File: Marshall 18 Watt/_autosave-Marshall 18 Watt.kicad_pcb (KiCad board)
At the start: 2 copper layers, 37 parts, among them J1 LOW, J2 HIGH, J3 Conn_01x03_Socket, J4 Heater, U1 ECC83, U2 ECC83, U3 EL84, U4 EL84

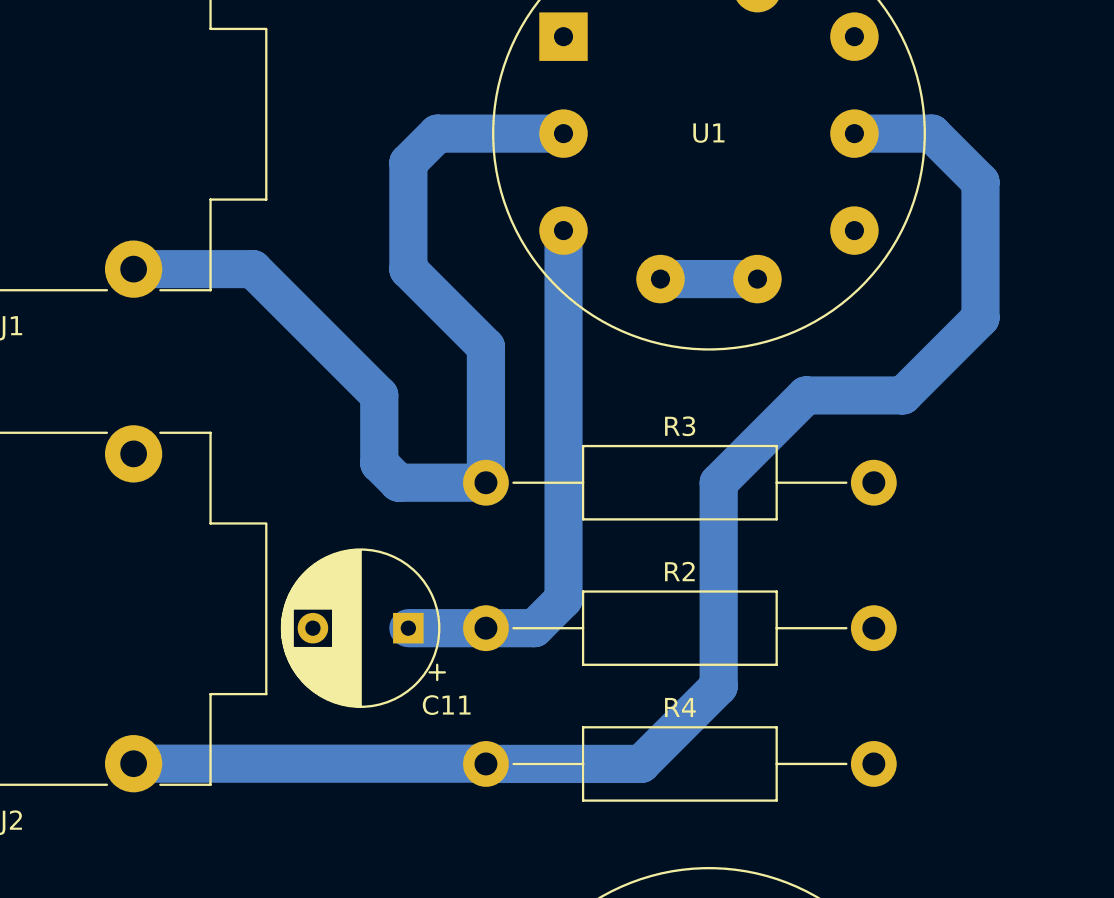
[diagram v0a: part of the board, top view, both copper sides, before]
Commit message: Update 11_03_25
add fender champ
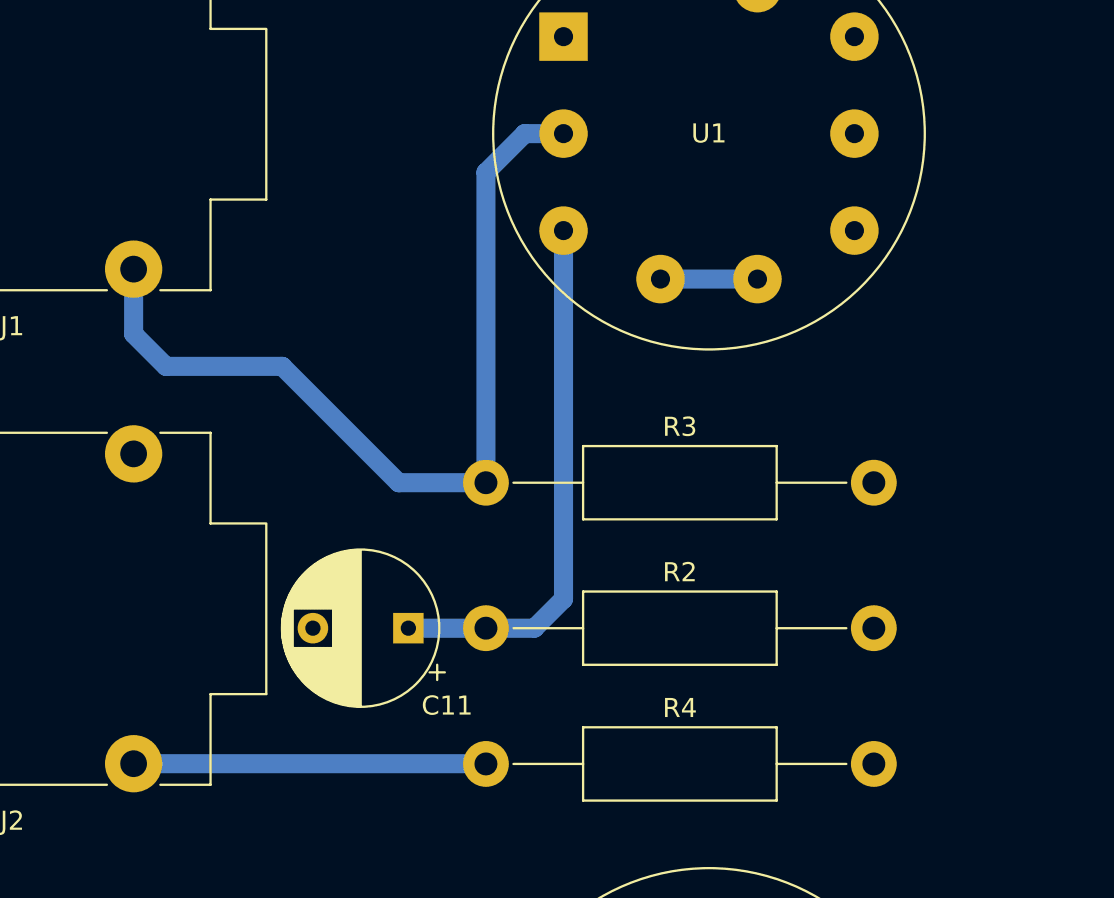
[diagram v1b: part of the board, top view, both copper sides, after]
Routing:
- net Net-(U1A-G): track 75.1 -> 18.5 mm
- net Net-(U1B-G): track 52.4 -> 46.2 mm
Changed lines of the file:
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@@
     )
   )
-  (segment (start 63.5 52.324) (end 66.04 52.324) (width 2) (layer "B.Cu") (net 6))
-  (segment (start 66.04 52.324) (end 67.564 50.8) (width 2) (layer "B.Cu") (net 6))
-  (segment (start 59.436 52.324) (end 63.5 52.324) (width 2) (layer "B.Cu") (net 6))
-  (segment (start 67.564 50.8) (end 67.564 31.496) (width 2) (layer "B.Cu") (net 6))
-  (segment (start 51.295 33.515) (end 57.912 40.132) (width 2) (layer "B.Cu") (net 10))
-  (segment (start 60.96 26.416) (end 67.564 26.416) (width 2) (layer "B.Cu") (net 10))
-  (segment (start 58.928 44.704) (end 63.5 44.704) (width 2) (layer "B.Cu") (net 10))
-  (segment (start 59.436 33.528) (end 59.436 27.94) (width 2) (layer "B.Cu") (net 10))
-  (segment (start 57.912 43.688) (end 58.928 44.704) (width 2) (layer "B.Cu") (net 10))
-  (segment (start 57.912 40.132) (end 57.912 43.688) (width 2) (layer "B.Cu") (net 10))
-  (segment (start 59.436 27.94) (end 60.96 26.416) (width 2) (layer "B.Cu") (net 10))
-  (segment (start 63.5 44.704) (end 63.5 37.592) (width 2) (layer "B.Cu") (net 10))
-  (segment (start 63.5 37.592) (end 59.436 33.528) (width 2) (layer "B.Cu") (net 10))
-  (segment (start 45.043 33.515) (end 51.295 33.515) (width 2) (layer "B.Cu") (net 10))
-  (segment (start 71.628 59.436) (end 75.692 55.372) (width 2) (layer "B.Cu") (net 11))
-  (segment (start 85.344 40.132) (end 89.408 36.068) (width 2) (layer "B.Cu") (net 11))
-  (segment (start 75.692 44.704) (end 80.264 40.132) (width 2) (layer "B.Cu") (net 11))
-  (segment (start 80.264 40.132) (end 85.344 40.132) (width 2) (layer "B.Cu") (net 11))
-  (segment (start 86.868 26.416) (end 82.804 26.416) (width 2) (layer "B.Cu") (net 11))
-  (segment (start 63.487 59.423) (end 63.5 59.436) (width 2) (layer "B.Cu") (net 11))
-  (segment (start 89.408 28.956) (end 86.868 26.416) (width 2) (layer "B.Cu") (net 11))
-  (segment (start 89.408 36.068) (end 89.408 28.956) (width 2) (layer "B.Cu") (net 11))
-  (segment (start 45.043 59.423) (end 63.487 59.423) (width 2) (layer "B.Cu") (net 11))
-  (segment (start 63.5 59.436) (end 71.628 59.436) (width 2) (layer "B.Cu") (net 11))
-  (segment (start 75.692 55.372) (end 75.692 44.704) (width 2) (layer "B.Cu") (net 11))
-  (segment (start 72.644 34.036) (end 77.724 34.036) (width 2) (layer "B.Cu") (net 19))
+  (segment (start 63.5 52.324) (end 59.436 52.324) (width 1) (layer "B.Cu") (net 6))
+  (segment (start 67.564 50.8) (end 67.564 31.496) (width 1) (layer "B.Cu") (net 6))
+  (segment (start 63.5 52.324) (end 66.04 52.324) (width 1) (layer "B.Cu") (net 6))
+  (segment (start 66.04 52.324) (end 67.564 50.8) (width 1) (layer "B.Cu") (net 6))
+  (segment (start 46.736 38.608) (end 52.832 38.608) (width 1) (layer "B.Cu") (net 10))
+  (segment (start 58.928 44.704) (end 63.5 44.704) (width 1) (layer "B.Cu") (net 10))
+  (segment (start 65.532 26.416) (end 67.564 26.416) (width 1) (layer "B.Cu") (net 10))
+  (segment (start 63.5 44.704) (end 63.5 28.448) (width 1) (layer "B.Cu") (net 10))
+  (segment (start 52.832 38.608) (end 58.928 44.704) (width 1) (layer "B.Cu") (net 10))
+  (segment (start 63.5 28.448) (end 65.532 26.416) (width 1) (layer "B.Cu") (net 10))
+  (segment (start 45.043 36.915) (end 46.736 38.608) (width 1) (layer "B.Cu") (net 10))
+  (segment (start 45.043 33.515) (end 45.043 36.915) (width 1) (layer "B.Cu") (net 10))
+  (segment (start 45.043 59.423) (end 63.487 59.423) (width 1) (layer "B.Cu") (net 11))
+  (segment (start 63.487 59.423) (end 63.5 59.436) (width 1) (layer "B.Cu") (net 11))
+  (segment (start 72.644 34.036) (end 77.724 34.036) (width 1) (layer "B.Cu") (net 19))
 )
